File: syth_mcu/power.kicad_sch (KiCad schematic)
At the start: 24 parts, among them U4 AMS1117-3.3

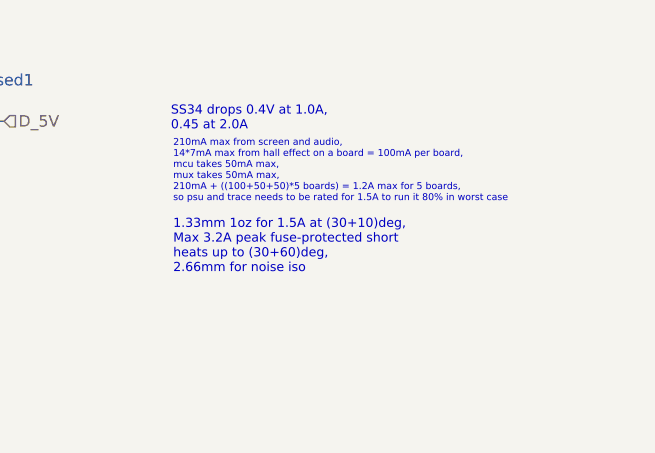
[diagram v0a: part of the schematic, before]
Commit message: System check, DRC runs
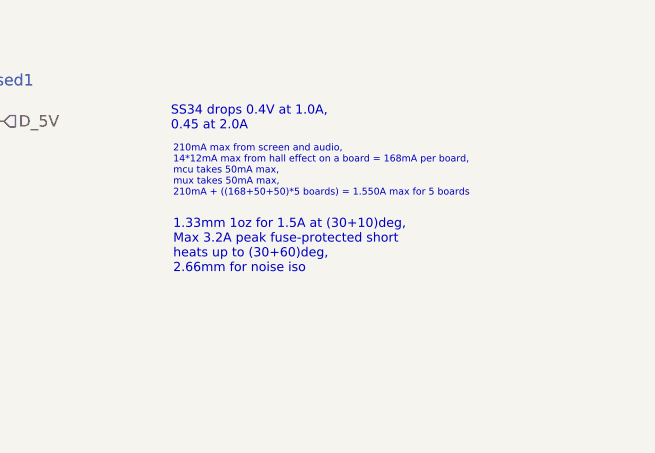
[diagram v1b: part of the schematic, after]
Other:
- note added: "210mA max from screen and audio, 14*12mA max from hall effect on a board = 168mA per board, mcu takes 50mA max, mux takes 50mA max, 210mA + ((168+50+50)*5 boards) = 1.550A max for 5 boards"
- note removed: "210mA max from screen and audio, 14*7mA max from hall effect on a board = 100mA per board, mcu takes 50mA max, mux takes 50mA max, 210mA + ((100+50+50)*5 boards) = 1.2A max for 5 boards, so psu and trace needs to be rated for 1.5A to run it 80% in worst case"
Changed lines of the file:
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@@
 		)
 	)
-	(text "210mA max from screen and audio,\n14*7mA max from hall effect on a board = 100mA per board,\nmcu takes 50mA max,\nmux takes 50mA max,\n210mA + ((100+50+50)*5 boards) = 1.2A max for 5 boards,\nso psu and trace needs to be rated for 1.5A to run it 80% in worst case"
+	(text "210mA max from screen and audio,\n14*12mA max from hall effect on a board = 168mA per board,\nmcu takes 50mA max,\nmux takes 50mA max,\n210mA + ((168+50+50)*5 boards) = 1.550A max for 5 boards"
 		(exclude_from_sim no)
 		(at 147.066 32.258 0)
